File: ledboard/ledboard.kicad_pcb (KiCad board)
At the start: 2 copper layers, 86 x 57.2 mm, 58 parts, among them J1 LEFT, J2 PWR_L, J3 RIGHT, J4 PWR_R, J5 Conn_01x03_Male, J6 Conn_01x02_Male, J7 Conn_02x20_Odd_Even, J8 Conn_01x02_Shielded, M1 MPMOS, U1 AL8860, U2 AL8860, U3 LM22676MR-5

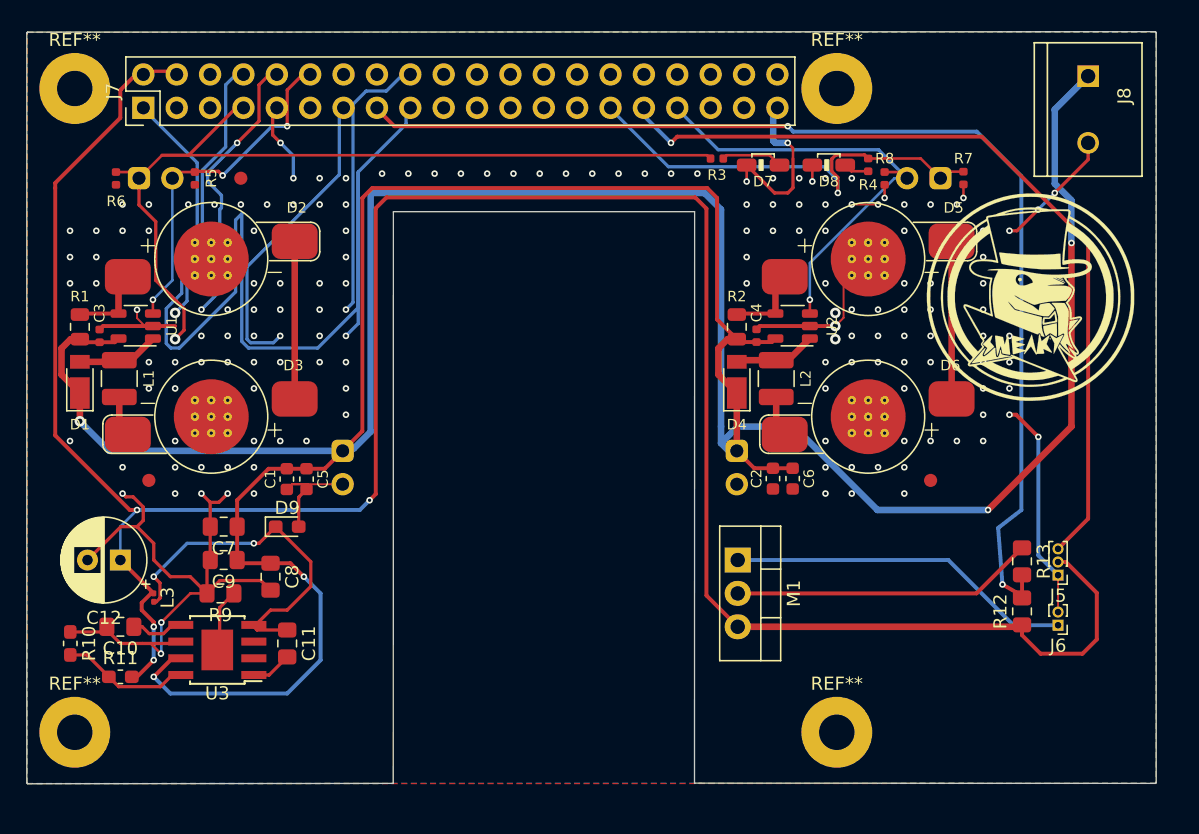
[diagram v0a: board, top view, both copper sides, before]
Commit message: Umarım son olur
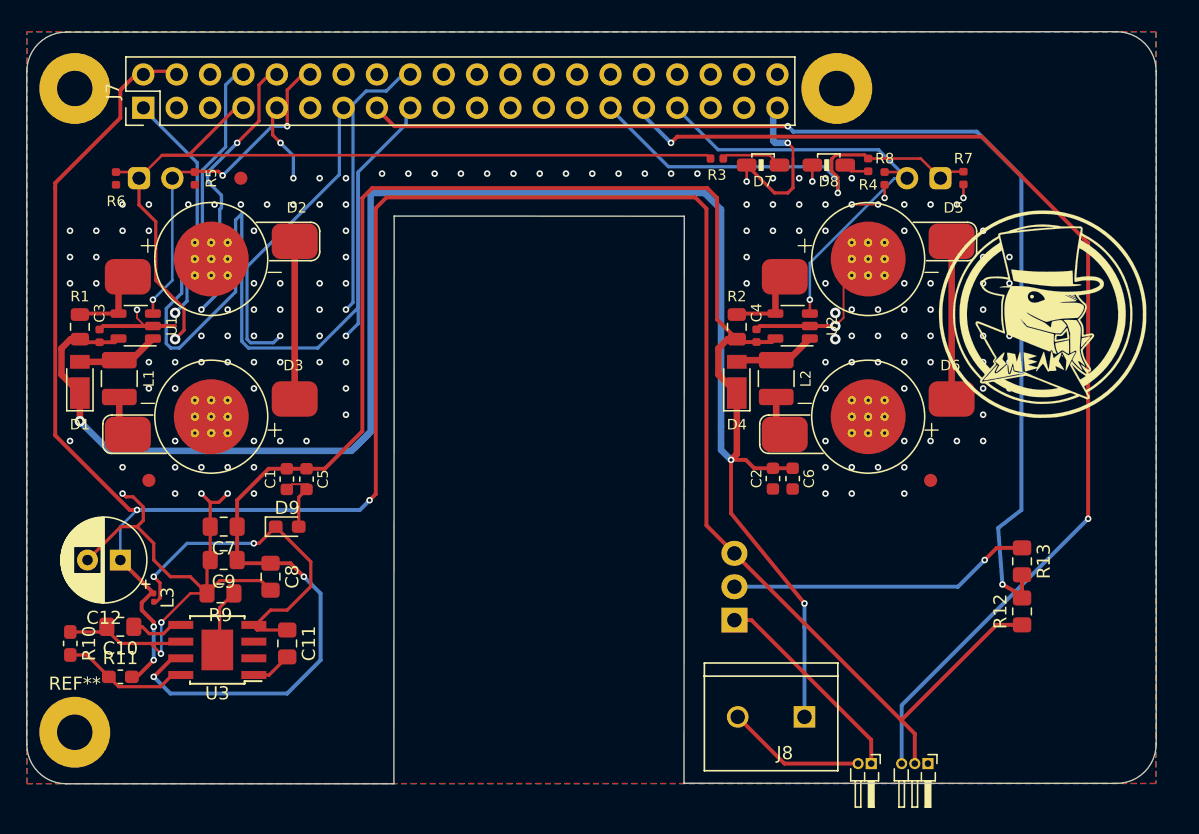
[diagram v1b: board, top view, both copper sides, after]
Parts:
- removed J2: PWR_L, ledboard:PinHeader_1x02_P2.54mm_Vertical_RoundRect
- removed J4: PWR_R, ledboard:PinHeader_1x02_P2.54mm_Vertical_RoundRect
- removed the REF** at (92.6, 84.4)
- J5: footprint Connector_PinHeader_1.00mm:PinHeader_1x03_P1.00mm_Vertical -> Connector_PinHeader_1.00mm:PinHeader_1x03_P1.00mm_Horizontal
- J6: footprint Connector_PinHeader_1.00mm:PinHeader_1x02_P1.00mm_Vertical -> Connector_PinHeader_1.00mm:PinHeader_1x02_P1.00mm_Horizontal
- M1: moved to B.Cu
- moved J8 52.1 mm to (87.6, 83.2), turned to 180 degrees
- moved J6 17.7 mm to (95.2, 86.8), turned to 270 degrees
- moved J5 17.4 mm to (99.5, 86.8), turned to 270 degrees
- moved M1 4.58 mm to (84.8, 75.9), turned to 90 degrees
- moved G*** 1.59 mm to (108.3, 52.6)
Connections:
- J7 pad 4: +5V -> (no net)
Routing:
- net +12V: track 280.0 -> 243.9 mm
- net /PWM_LED: track 63.4 -> 84.7 mm, vias 1 -> 2
- net GND: track 122.4 -> 102.2 mm, vias 152 -> 147
- net Net-(J6-Pad1): track 26.4 -> 16.0 mm
- net +5V: track 193.3 -> 185.1 mm
- net Net-(M1-Pad2): vias 0 -> 1
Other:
- outline, holes or cut-outs redrawn

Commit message: Kicadden nefret ediyorum
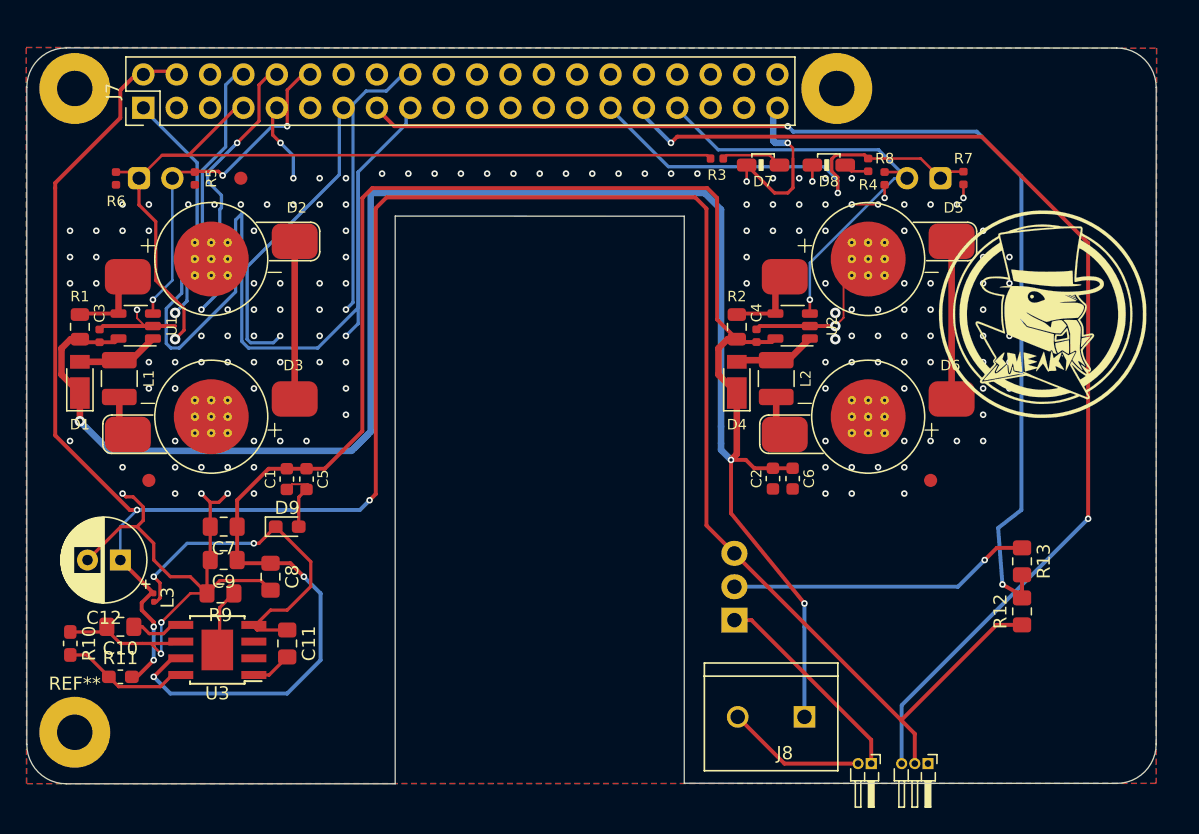
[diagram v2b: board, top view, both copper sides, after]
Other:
- board size 86 x 57.2 mm -> 86 x 56 mm

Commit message: power soket
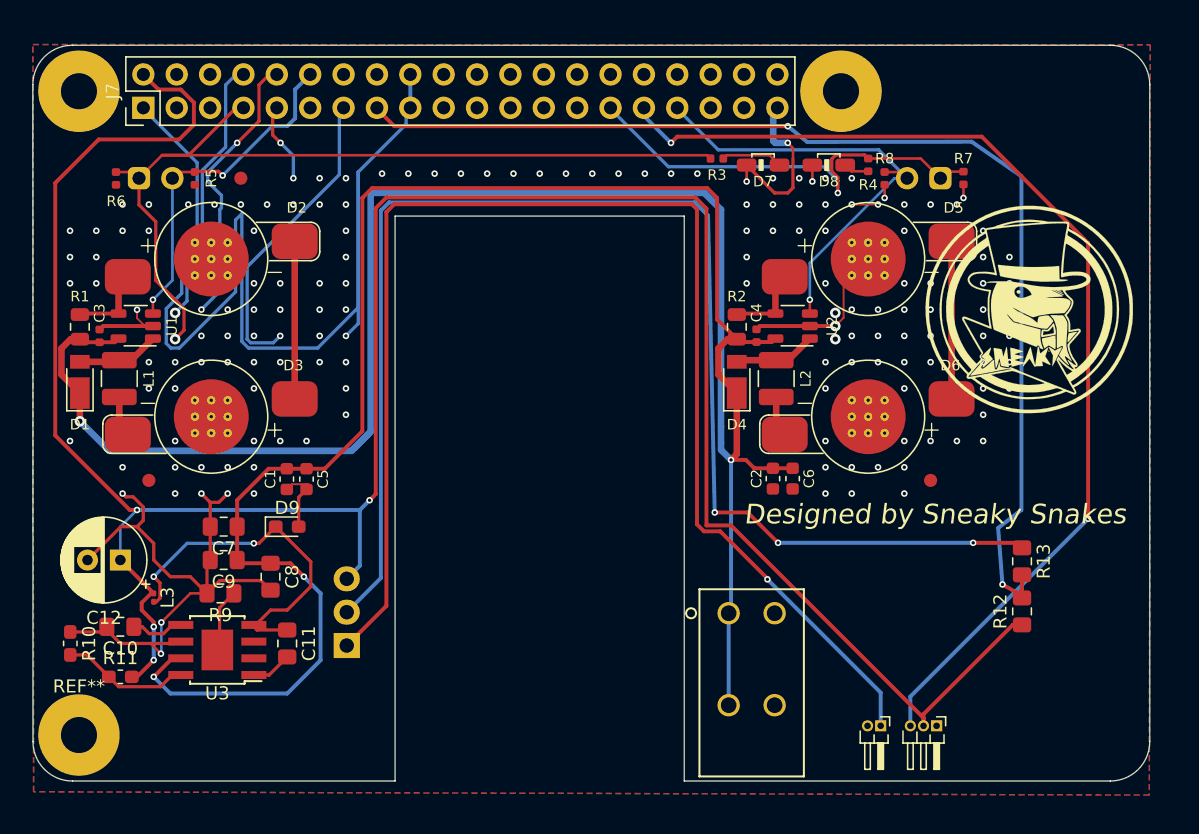
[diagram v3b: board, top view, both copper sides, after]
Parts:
- removed J8: Conn_01x02_Shielded, Connector:TE_282837-2
- removed the REF** at (34.6, 84.4)
- removed the REF** at (92.6, 35.4)
- removed the REF** at (34.6, 35.4)
- added J2: 1824420000, footprints:1824420000, F.Cu at (84.4, 75.4)
- added REF**: MountingHole_2.7mm_M2.5_Pad, MountingHole:MountingHole_2.7mm_M2.5_Pad, F.Cu at (92.9, 35.6)
- added REF**: MountingHole_2.7mm_M2.5_Pad, MountingHole:MountingHole_2.7mm_M2.5_Pad, F.Cu at (34.9, 84.6)
- added REF**: MountingHole_2.7mm_M2.5_Pad, MountingHole:MountingHole_2.7mm_M2.5_Pad, F.Cu at (34.9, 35.6)
- moved M1 29.6 mm to (55.3, 77.8)
- moved J6 2.96 mm to (96.0, 83.9)
- moved J5 2.95 mm to (100.2, 83.9)
- moved G*** 1.08 mm to (107.3, 52.2)
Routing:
- net Net-(J6-Pad1): track 16.0 -> 104.2 mm, vias 0 -> 1
- net Net-(M1-Pad2): track 23.1 -> 104.3 mm, vias 1 -> 3
- net (no net): track 177.0 -> 158.6 mm
- net GND: track 102.2 -> 89.9 mm
- net +5V: track 185.1 -> 193.4 mm
- net /PWM_LED: track 84.7 -> 81.6 mm
- net +12V: track 243.9 -> 241.3 mm, vias 5 -> 4
- net /CTRL_L: track 26.3 -> 26.2 mm, vias 3 -> 2
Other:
- board size 86 x 56 mm -> 85 x 56 mm
- board text added: "Designed by Sneaky Snakes"
